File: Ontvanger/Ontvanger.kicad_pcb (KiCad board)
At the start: 2 copper layers, 30.5 x 20.3 mm, 4 parts, among them IC1 STM32WB30CEU5A, IC2 QAM-RX10-433, J1 Conn_01x04_Male, U1 BAT-HLD-001

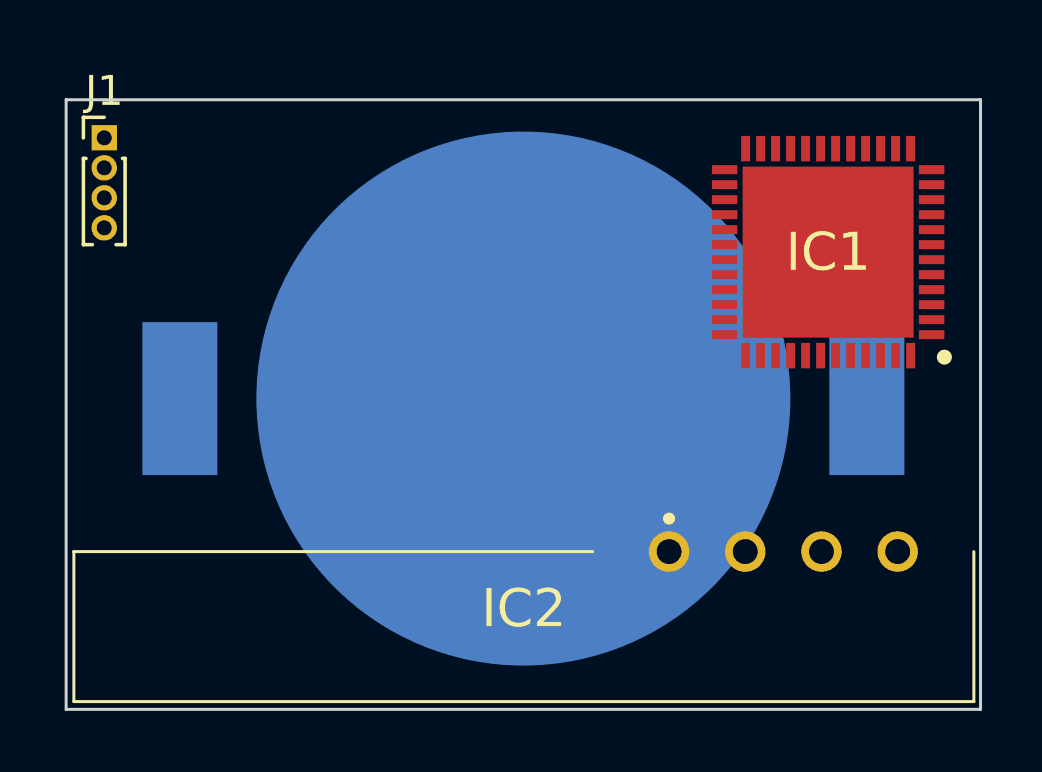
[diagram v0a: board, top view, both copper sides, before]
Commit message: filss added
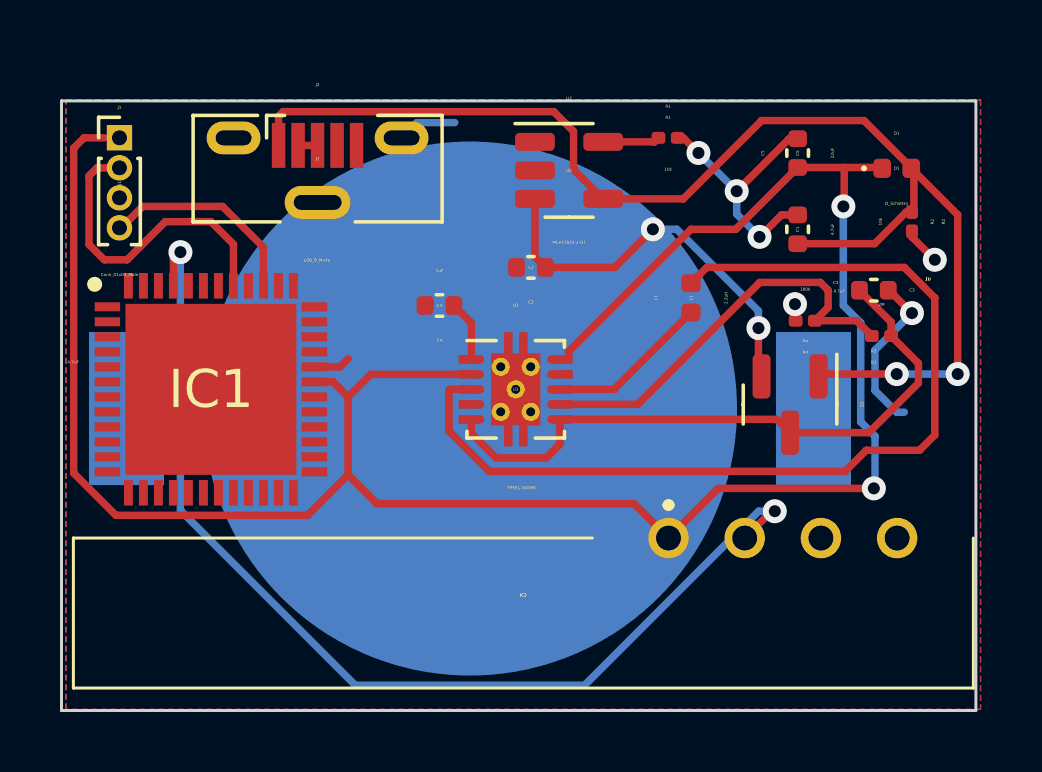
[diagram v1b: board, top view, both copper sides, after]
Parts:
- added C1: 4.7uF, Capacitor_SMD:C_0402_1005Metric, F.Cu at (181.9, 89.4)
- added C2: 4.7uF, Capacitor_SMD:C_0402_1005Metric, F.Cu at (173.0, 90.7)
- added C3: 4.7uF, Capacitor_SMD:C_0402_1005Metric, F.Cu at (184.4, 91.4)
- added C4: 1uF, Capacitor_SMD:C_0402_1005Metric, F.Cu at (169.9, 91.9)
- added C5: 22uF, Capacitor_SMD:C_0402_1005Metric, F.Cu at (181.9, 86.9)
- added D1: D_Schottky, Diode_SMD:D_0402_1005Metric, F.Cu at (185.2, 87.4)
- added J2: USB_B_Micro, Connector_USB:USB_Micro-B_Molex-105133-0001, F.Cu at (165.9, 87.4)
- added L1: 2.2uH, Inductor_SMD:L_0402_1005Metric, F.Cu at (178.3, 91.7)
- added Q1: AO3401A, Package_TO_SOT_SMD:SOT-23, F.Cu at (181.6, 95.2)
- added R1: 10k, Resistor_SMD:R_0201_0603Metric, F.Cu at (177.5, 86.4)
- added R2: 10k, Resistor_SMD:R_0201_0603Metric, F.Cu at (185.7, 89.2)
- added R3: 2M, Resistor_SMD:R_0201_0603Metric, F.Cu at (184.7, 93.0)
- added R4: 180k, Resistor_SMD:R_0201_0603Metric, F.Cu at (182.1, 92.5)
- added U2: MCP73831-2-OT, Package_TO_SOT_SMD:SOT-23-5, F.Cu at (174.2, 87.4)
- added U3: TPS61200DRC, Package_SON:Texas_S-PVSON-N10_ThermalVias, F.Cu at (172.5, 94.7)
- IC1: footprint SamacSys_Parts:QFN50P700X700X60-49N-D -> KiCad libs:QFN50P700X700X60-49N-D
- IC2: footprint SamacSys_Parts:QAMRX10433 -> KiCad libs:QAMRX10433
- U1: footprint SamacSys_Parts:BATHLD001 -> KiCad libs:BATHLD001
- moved IC1 21.1 mm to (162.3, 94.7), turned to 0 degrees
- moved U1 1.81 mm to (170.9, 95.4)
- moved J1 0.51 mm to (159.3, 86.4)
- moved IC2 0.45 mm to (177.6, 99.7)
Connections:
- IC1 pad 31: unconnected-(IC1-Pad31) -> 3V
- IC1 pad 32: Net-(IC1-Pad32) -> GND
- IC2 pad 1: Net-(IC1-Pad32) -> 3V
- IC2 pad 4: Net-(IC2-Pad4) -> GND
- J1 pad 1: Net-(IC1-Pad32) -> 3V
- J1 pad 3: Net-(IC2-Pad4) -> GND
- U1 pad 1: Net-(IC2-Pad4) -> GND
- U1 pad 2: unconnected-(U1-Pad2) -> GND
- U1 pad 3: Net-(IC1-Pad32) -> Net-(C2-Pad1)
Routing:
- net 3V: track 0.00 -> 73.9 mm, vias 0 -> 2
- net Net-(C1-Pad1): track 0.00 -> 43.8 mm, vias 0 -> 2
- net Net-(IC1-Pad45): track 0.00 -> 35.8 mm, vias 0 -> 2
- net Net-(L1-Pad2): track 0.00 -> 32.7 mm
- net Net-(C3-Pad1): track 0.00 -> 26.7 mm
- net GND: track 0.00 -> 19.4 mm, vias 0 -> 6
- net Net-(R3-Pad2): track 0.00 -> 13.8 mm
- net Net-(C2-Pad1): track 0.00 -> 13.4 mm, vias 0 -> 2
- net Net-(IC1-Pad41): track 0.00 -> 10.7 mm
- net Net-(IC1-Pad39): track 0.00 -> 6.94 mm
- net Net-(C4-Pad1): track 0.00 -> 2.04 mm
- net Net-(R1-Pad1): track 0.00 -> 1.90 mm
- net Net-(J2-Pad2): track 0.00 -> 0.65 mm
- added copper zone on B.Cu, net GND
- added copper zone on F.Cu, net GND
